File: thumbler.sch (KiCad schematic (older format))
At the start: 255 parts, among them J1 USB_B_Micro, J2 Conn_01x04, J3 Conn_01x04, J4 DIN-5_180degree, J5 Conn_01x04, J6 DIN-5_180degree, J7 Conn_01x04, J8 USB_B_Micro, SW1 SW_Push, SW2 SW_DIP_x05, SW3 SW_Push, SW4 SW_DIP_x05, U1 STM32F072C8Tx, U2 MCP1700-3302E_SOT89, U3 MCP1700-3302E_SOT89, U4 STM32F072C8Tx, X1 ENCODER_ANO

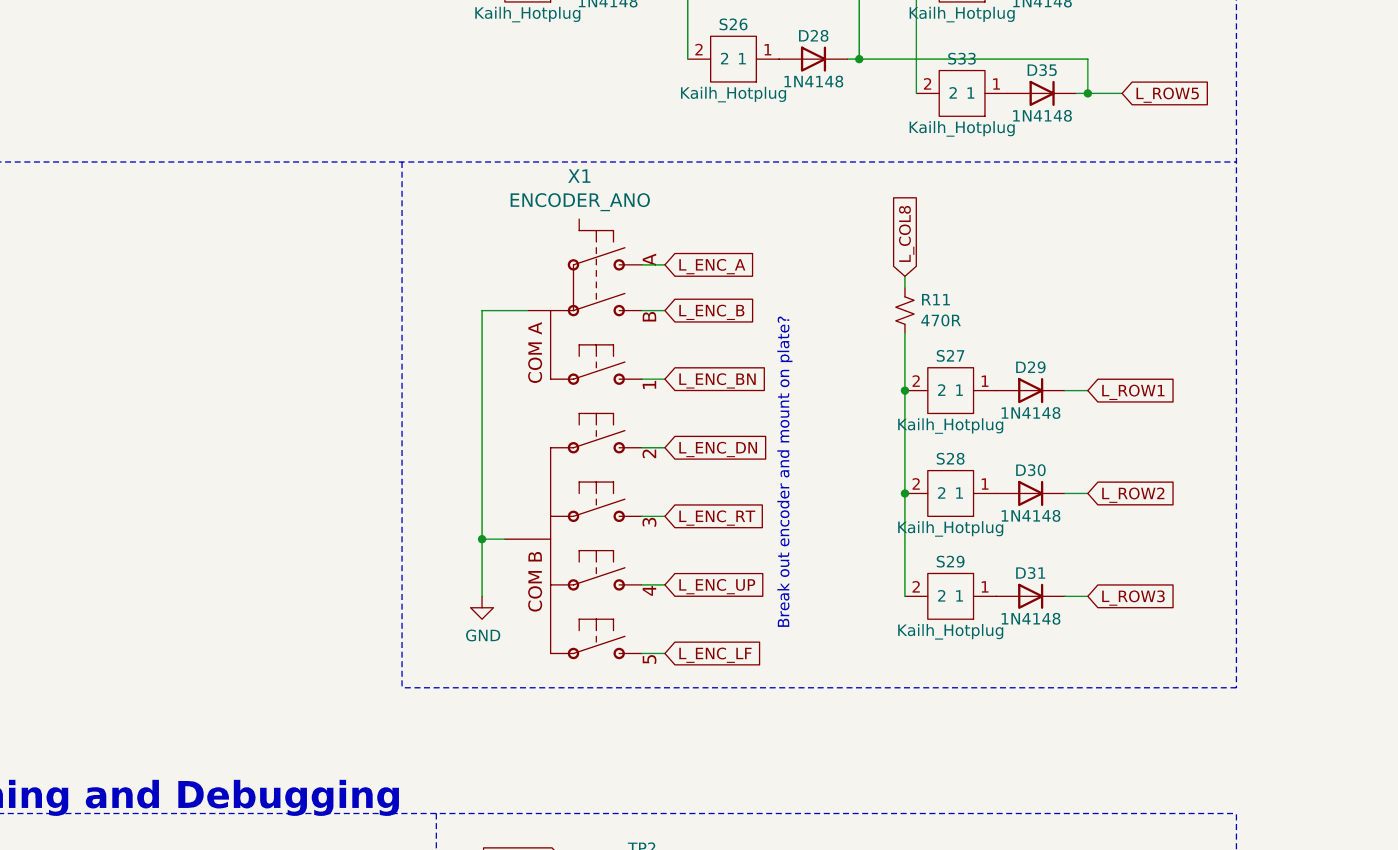
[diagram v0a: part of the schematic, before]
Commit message: 70 key laid out
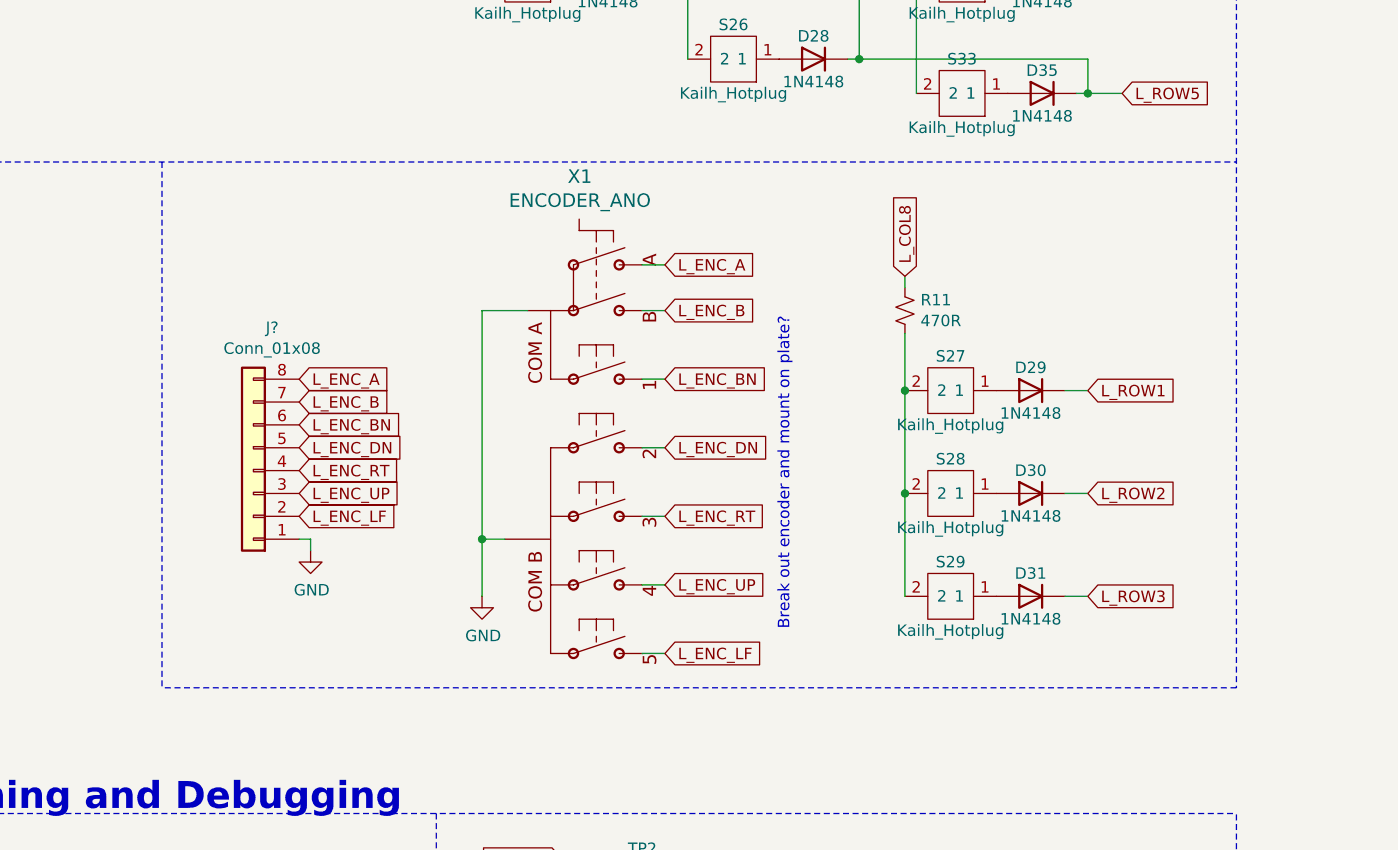
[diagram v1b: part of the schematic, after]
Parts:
- added J?: Conn_01x08, symbol Connector_Generic:Conn_01x08
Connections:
- net GND: now also J?.1 (Pin_1)
- net L_ENC_A: now also J?.8 (Pin_8)
- net L_ENC_B: now also J?.7 (Pin_7)
- net L_ENC_BN: now also J?.6 (Pin_6)
- net L_ENC_DN: now also J?.5 (Pin_5)
- net L_ENC_LF: now also J?.2 (Pin_2)
- net L_ENC_RT: now also J?.4 (Pin_4)
- net L_ENC_UP: now also J?.3 (Pin_3)
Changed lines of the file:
@@
 	9750 10100 9750 10150
 Wire Notes Line
-	11200 11900 7550 11900
-Wire Notes Line
-	7550 9600 7550 11900
+	6500 9600 6500 11900
 Wire Notes Line
 	11200 5550 11200 11900
@@
 	19100 8200 19100 8700
 Connection ~ 19100 8200
+$Comp
+L Connector_Generic:Conn_01x08 J?
+U 1 1 6D7D2149
+P 6900 10950
+F 0 "J?" H 6818 10325 50  0000 C CNN
+F 1 "Conn_01x08" H 6818 10416 50  0000 C CNN
+F 2 "" H 6900 10950 50  0001 C CNN
+F 3 "~" H 6900 10950 50  0001 C CNN
+	1    6900 10950
+	-1   0    0    1
+$EndComp
+Text GLabel 7100 10550 2    50   Input ~ 0
+L_ENC_A
+Text GLabel 7100 10650 2    50   Input ~ 0
+L_ENC_B
+Text GLabel 7100 10750 2    50   Input ~ 0
+L_ENC_BN
+Text GLabel 7100 10850 2    50   Input ~ 0
+L_ENC_DN
+Text GLabel 7100 11050 2    50   Input ~ 0
+L_ENC_UP
+Text GLabel 7100 11150 2    50   Input ~ 0
+L_ENC_LF
+Text GLabel 7100 10950 2    50   Input ~ 0
+L_ENC_RT
+$Comp
+L power:GND #PWR?
+U 1 1 6DC33371
+P 7150 11300
+F 0 "#PWR?" H 7150 11050 50  0001 C CNN
+F 1 "GND" H 7155 11127 50  0000 C CNN
+F 2 "" H 7150 11300 50  0001 C CNN
+F 3 "" H 7150 11300 50  0001 C CNN
+	1    7150 11300
+	1    0    0    -1
+$EndComp
+Wire Wire Line
+	7100 11250 7150 11250
+Wire Wire Line
+	7150 11250 7150 11300
+Wire Notes Line
+	11200 11900 6500 11900
 $EndSCHEMATC
